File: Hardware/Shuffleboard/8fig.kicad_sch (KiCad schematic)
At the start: 22 parts

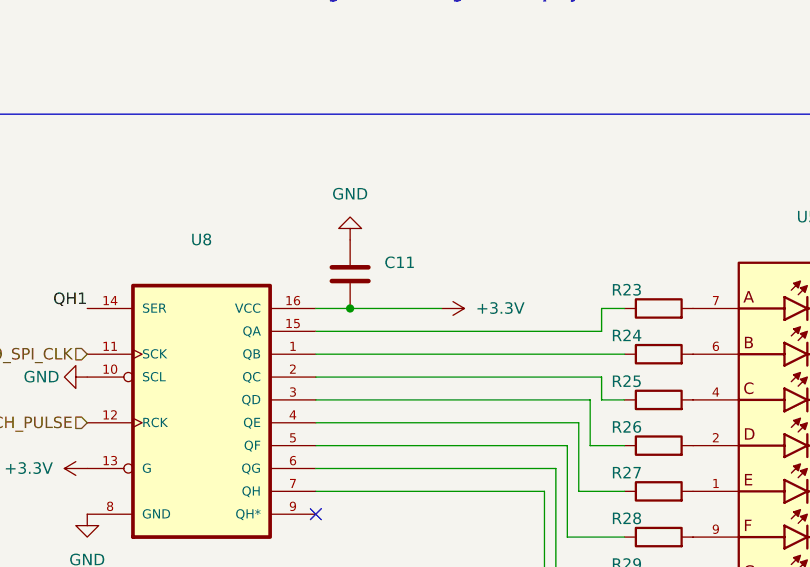
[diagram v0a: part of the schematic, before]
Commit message: finalized
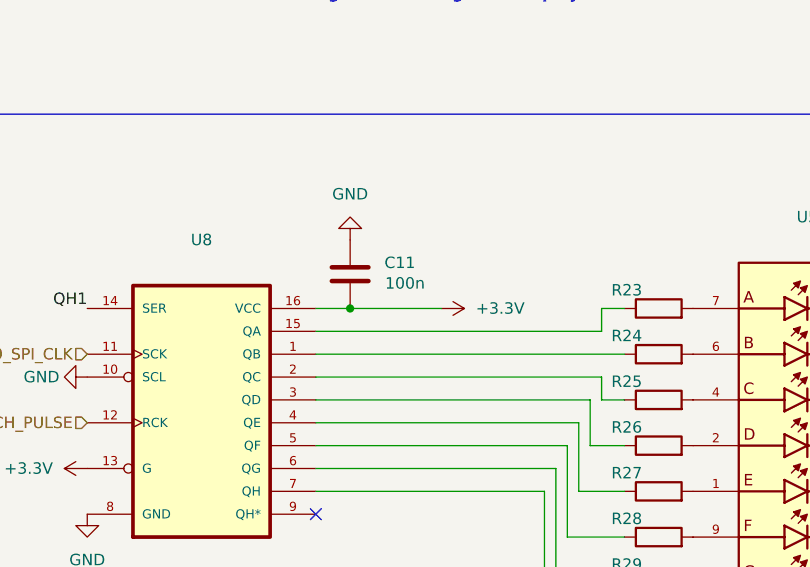
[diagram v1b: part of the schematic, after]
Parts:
- C11: value (none) -> 100n
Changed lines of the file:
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@@
 		(in_pos_files yes)
 		(dnp no)
-		(fields_autoplaced yes)
 		(property "Reference" "C11"
 			(at 68.58 101.5999 0)
@@
 			)
 		)
-		(property "Value" ""
-			(at 64.77 102.87 0)
-			(hide yes)
+		(property "Value" "100n"
+			(at 70.866 103.886 0)
 			(show_name no)
 			(do_not_autoplace no)
